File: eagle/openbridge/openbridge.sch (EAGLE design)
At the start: 5 parts, among them IC1 7805TV

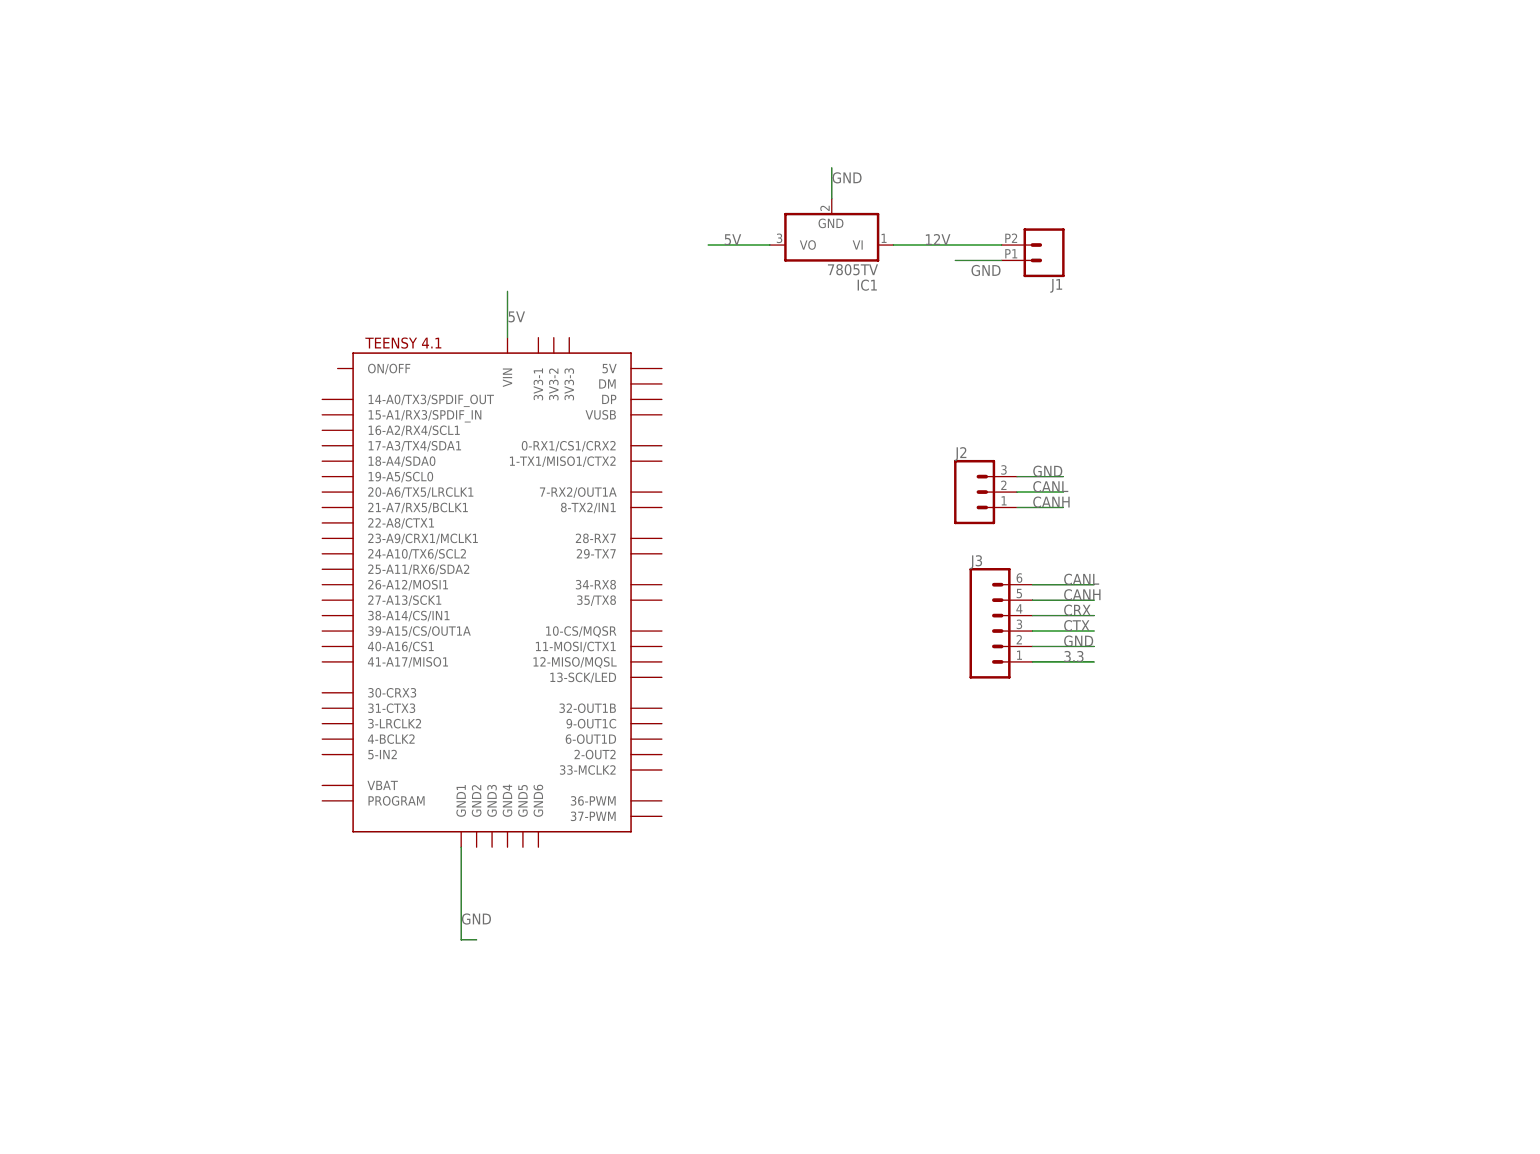
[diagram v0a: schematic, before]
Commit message: 2nd version
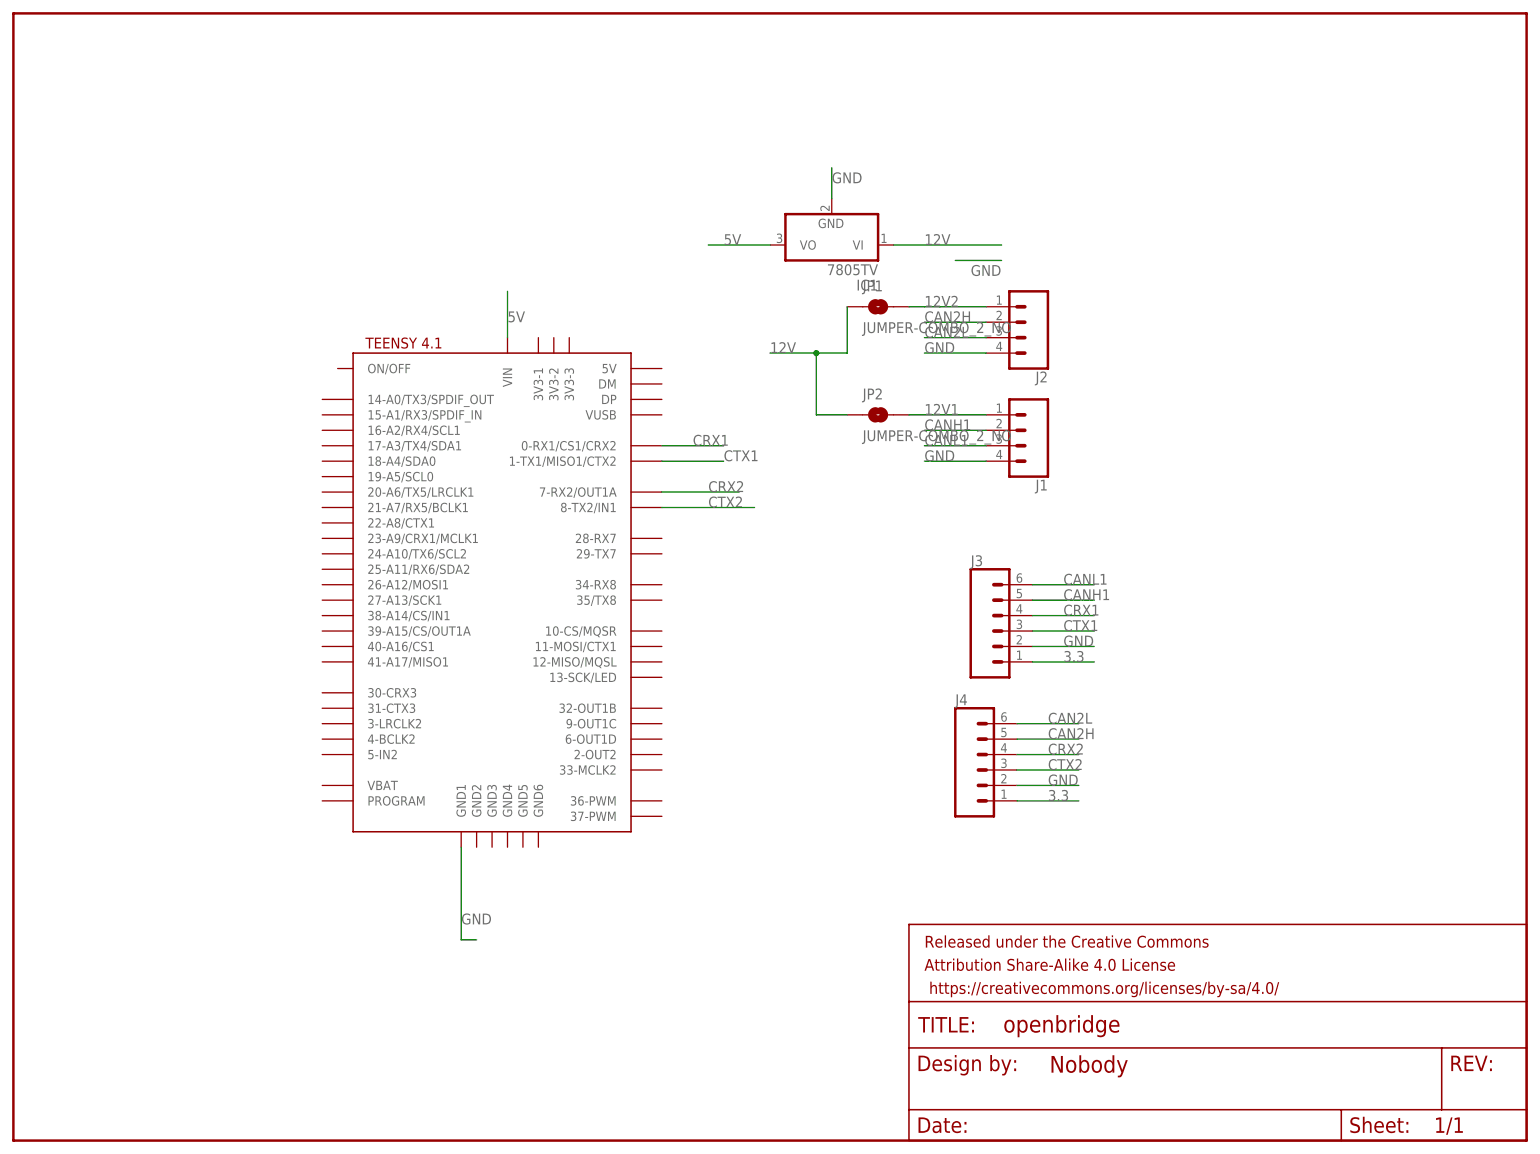
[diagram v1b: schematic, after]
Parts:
- added FRAME1: FRAME-LETTERNO_PACKAGE, SparkFun-Aesthetics:FRAME-LETTERNO_PACKAGE
- added J4: (no value), SparkFun-Connectors:CONN_06LONGPADS
- added JP1, JP2: JUMPER-COMBO_2_NO, SparkFun-Jumpers:JUMPER-COMBO_2_NO
- J1: device SparkFun-Connectors:CONN_02SCREWTERMINAL-6.35MM-2 -> SparkFun-Connectors:CONN_04SCREW
- J2: device SparkFun-Connectors:CONN_03-SCREW-5MM -> SparkFun-Connectors:CONN_04SCREW
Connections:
- removed net CANH: J2.1, J3.5
- removed net CANL: J2.2, J3.6
- removed net CRX: J3.4
- removed net CTX: J3.3
- new net 12V1: J1.1, JP2.2
- new net 12V2: J2.1, JP1.2
- new net CAN2H: J2.2, J4.5
- new net CAN2L: J2.3, J4.6
- new net CANH1: J1.2, J3.5
- new net CANL1: J1.3, J3.6
- new net CRX1: J3.4, U$1.0-RX1/CS1/CRX2
- new net CRX2: J4.4, U$1.7-RX2/OUT1A
- new net CTX1: J3.3, U$1.1-TX1/MISO1/CTX2
- new net CTX2: J4.3, U$1.8-TX2/IN1
- net 12V: now also JP1.1, JP2.1; no longer J1.1
- net 3.3: now also J4.1
- net GND: now also J1.4, J2.4, J4.2; no longer J1.2, J2.3
